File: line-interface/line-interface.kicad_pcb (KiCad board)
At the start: 2 copper layers, 80 x 49 mm, 35 parts, among them IC1 ATTINY441-SSU, J1 CONN_01X06, P1 CONN_02X03, P2 CONN_01X04, Q1 NDT2955, U1 LR12K, U2 SN65HVD72, X1 16MHz

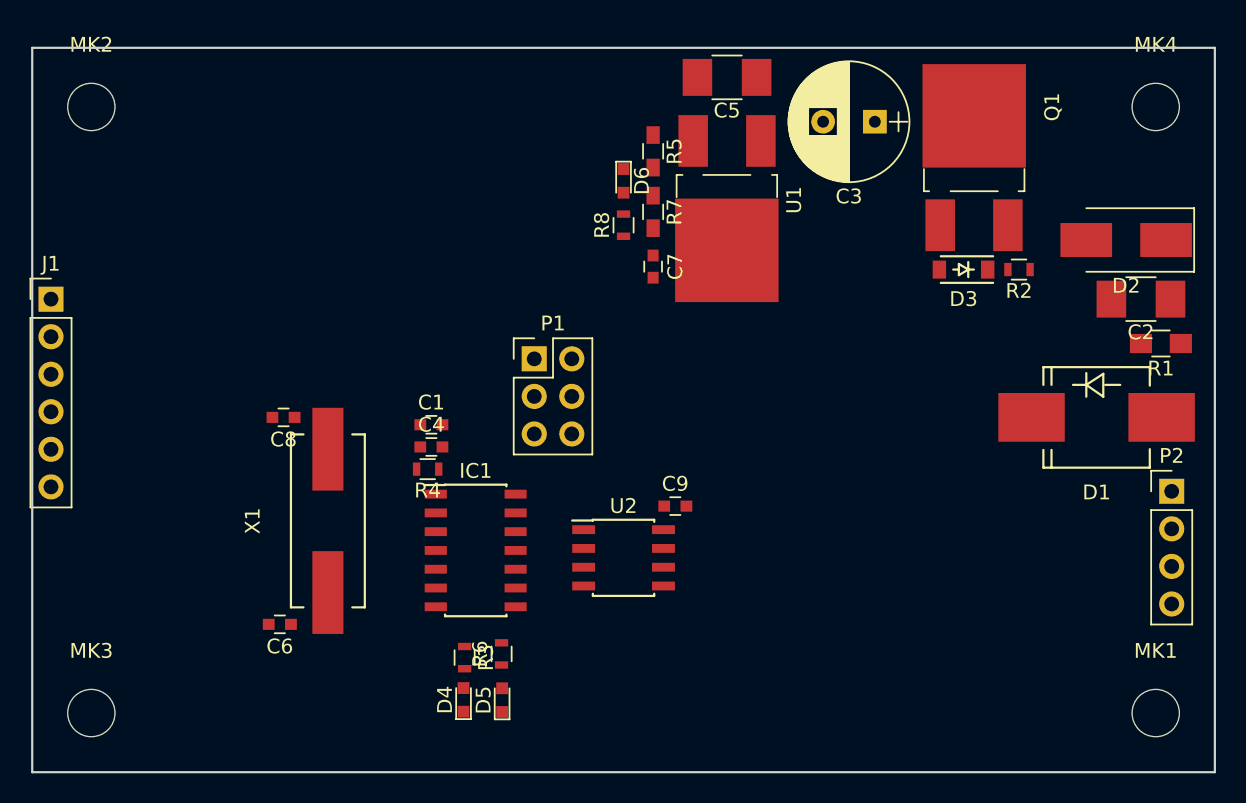
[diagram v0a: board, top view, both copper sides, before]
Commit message: Finish routing the board, manufacturing order sent
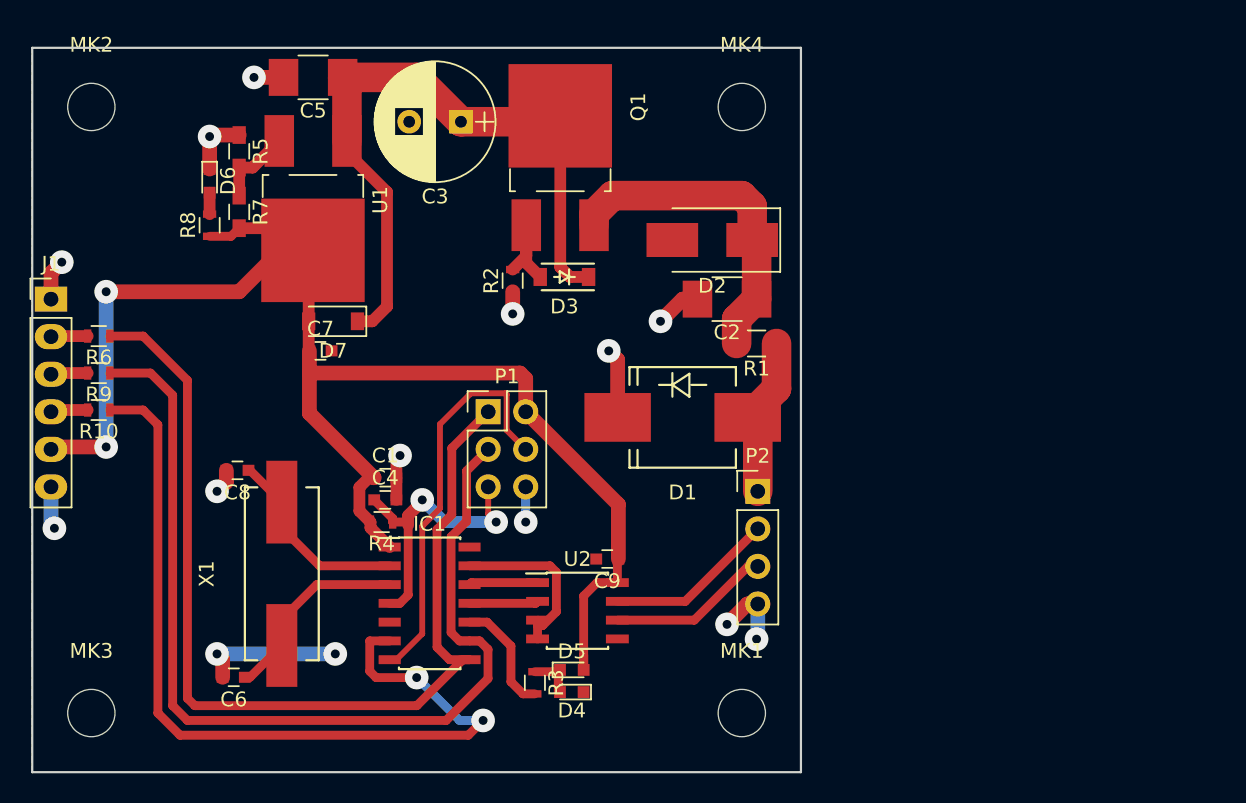
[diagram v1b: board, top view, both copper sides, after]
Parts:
- added D7: D, Diodes_SMD:D_SOD-123, F.Cu at (120.3, 118.5)
- added R10: 10k, Resistors_SMD:R_0603, F.Cu at (104.5, 124.5)
- added R9: 10k, Resistors_SMD:R_0603, F.Cu at (104.5, 122.0)
- moved R6 34.7 mm to (104.5, 119.5), turned to 180 degrees
- moved R2 34.3 mm to (132.5, 115.8), turned to 90 degrees
- moved C2 28.0 mm to (147.0, 117.0)
- moved C3 28.0 mm to (129.0, 105.0)
- moved C5 28.0 mm to (119.0, 102.0)
- moved D1 28.0 mm to (144.0, 125.0)
- moved D2 28.0 mm to (146.0, 113.0)
- moved D6 28.0 mm to (112.0, 109.0)
- moved MK1 28.0 mm to (148.0, 145.0)
- moved MK4 28.0 mm to (148.0, 104.0)
- moved P2 28.0 mm to (149.1, 130.0)
- moved Q1 28.0 mm to (135.7, 108.3)
- moved R5 28.0 mm to (114.0, 107.0)
- moved R7 28.0 mm to (114.0, 111.1)
- moved R8 28.0 mm to (112.0, 112.0)
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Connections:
- net /EXCITATION renamed Net-(IC1-Pad5)
- D5 pad 1: GND -> Net-(D4-Pad2)
- D5 pad 2: Net-(D5-Pad2) -> +5V
- IC1 pad 6: Net-(IC1-Pad6) -> /~CS
- P2 pad 2: /RS485A -> /RS485B
- P2 pad 3: /RS485B -> /RS485A
- R3 pad 2: Net-(IC1-Pad6) -> Net-(IC1-Pad10)
- R6 pad 1: Net-(D5-Pad2) -> /MISO
- R6 pad 2: Net-(IC1-Pad10) -> /SERIAL_DATA_IN
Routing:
- net +5V: track 0.00 -> 109.1 mm, vias 0 -> 2
- net /MISO: track 0.00 -> 68.5 mm
- net /SCK: track 0.00 -> 67.2 mm
- net /~CS: track 0.00 -> 58.6 mm, vias 0 -> 2
- net Net-(C3-Pad1): track 0.00 -> 47.7 mm
- net GND: track 0.00 -> 43.3 mm, vias 0 -> 14
- net /MOSI: track 0.00 -> 27.3 mm
- net Net-(C2-Pad1): track 0.00 -> 23.0 mm
- net /RESET: track 0.00 -> 19.7 mm, vias 0 -> 2
- net Net-(C6-Pad1): track 0.00 -> 13.4 mm
- net Net-(C8-Pad1): track 0.00 -> 13.3 mm
- net Net-(IC1-Pad13): track 0.00 -> 11.7 mm
- net /RS485B: track 0.00 -> 11.5 mm
- net VCC: track 0.00 -> 11.1 mm
- net /RS485A: track 0.00 -> 11.0 mm
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- added copper zone on B.Cu, net GND
- added copper zone on F.Cu, net GND
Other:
- board size 80 x 49 mm -> 52 x 49 mm
